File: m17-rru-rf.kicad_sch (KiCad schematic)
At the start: 0 parts

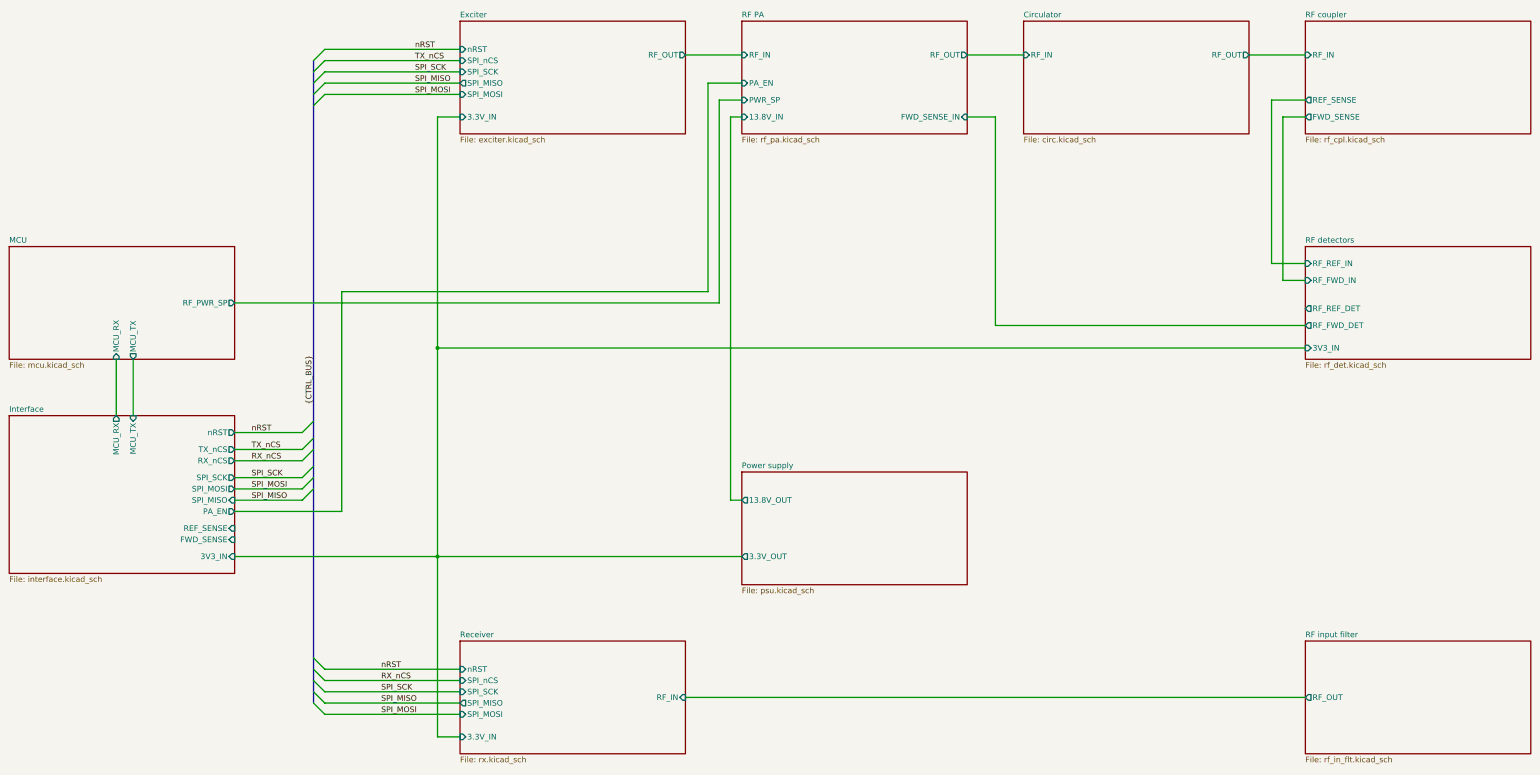
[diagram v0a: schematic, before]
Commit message: Add files via upload
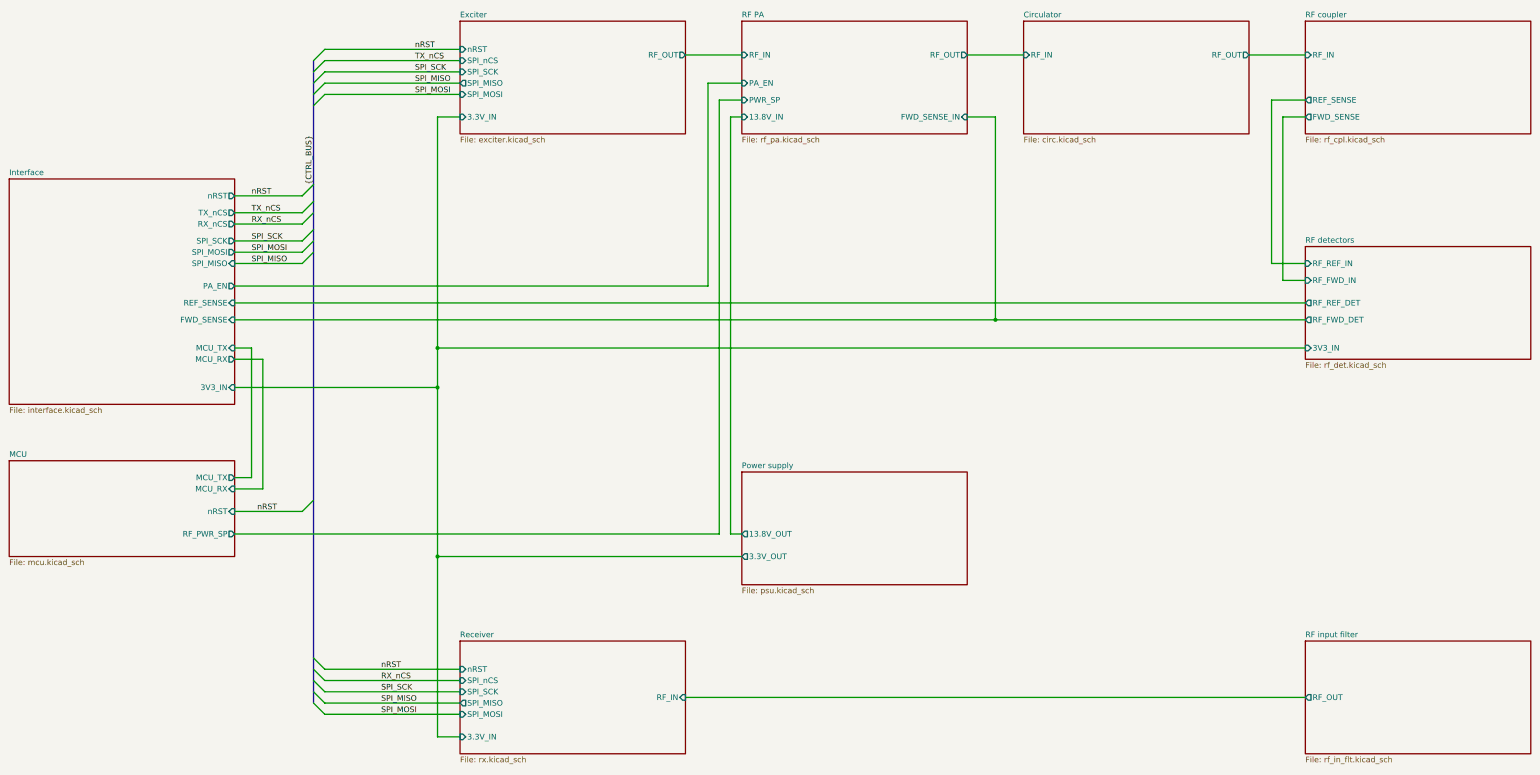
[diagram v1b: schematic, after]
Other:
- sheet MCU ports: added nRST; removed none
